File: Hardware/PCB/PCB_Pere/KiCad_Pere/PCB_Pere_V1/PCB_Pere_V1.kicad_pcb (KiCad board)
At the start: 4 copper layers, 52.9 x 80.1 mm, 88 parts, among them CN1 B2B-PH-K-S-GW, CN3 B4B-PH-K-S, CN4 B4B-PH-K-S, U2 TMC2209-LA-T, U3 Buck LMR51625, U4 8132H-10.000NL33DTL, U5 Buck LMR51625, U6 8132H-10.000NL33DTL, U7 TMC2209-LA-T

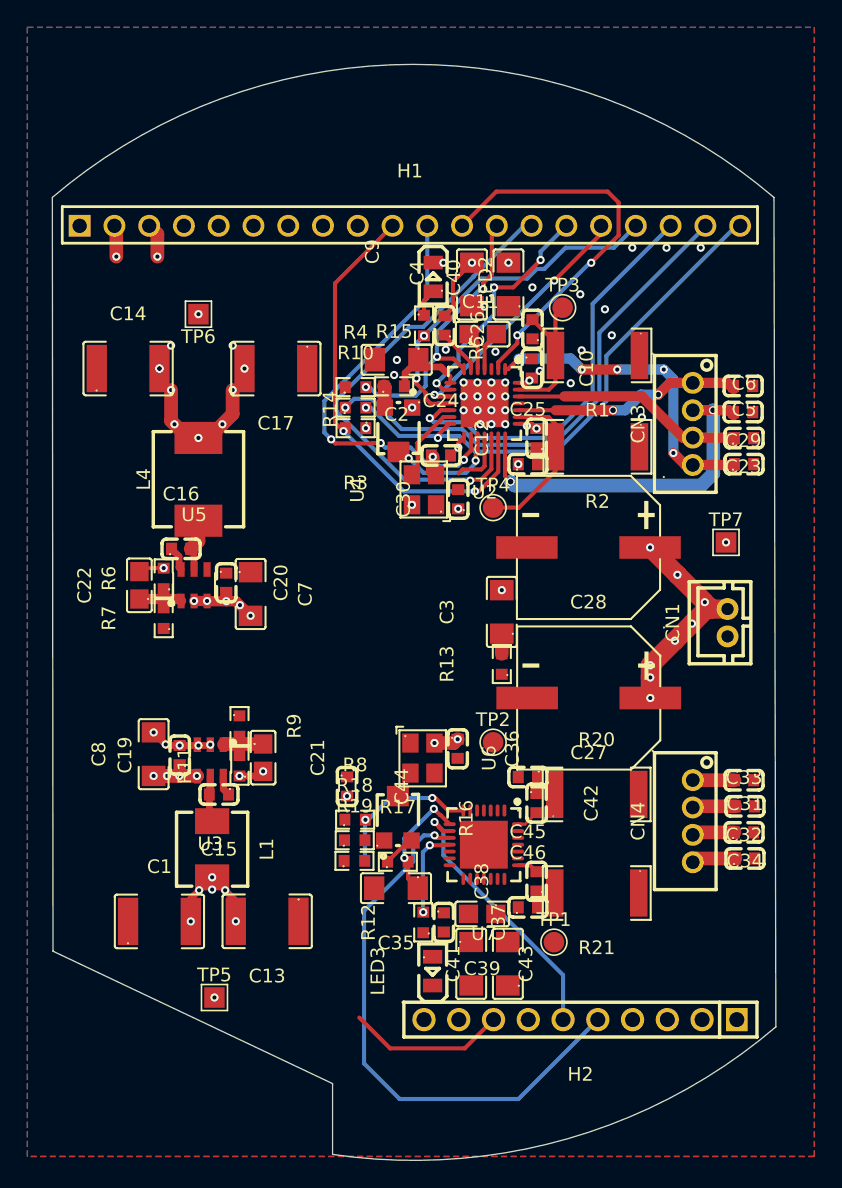
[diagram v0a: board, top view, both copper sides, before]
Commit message: pcb père quasi fini
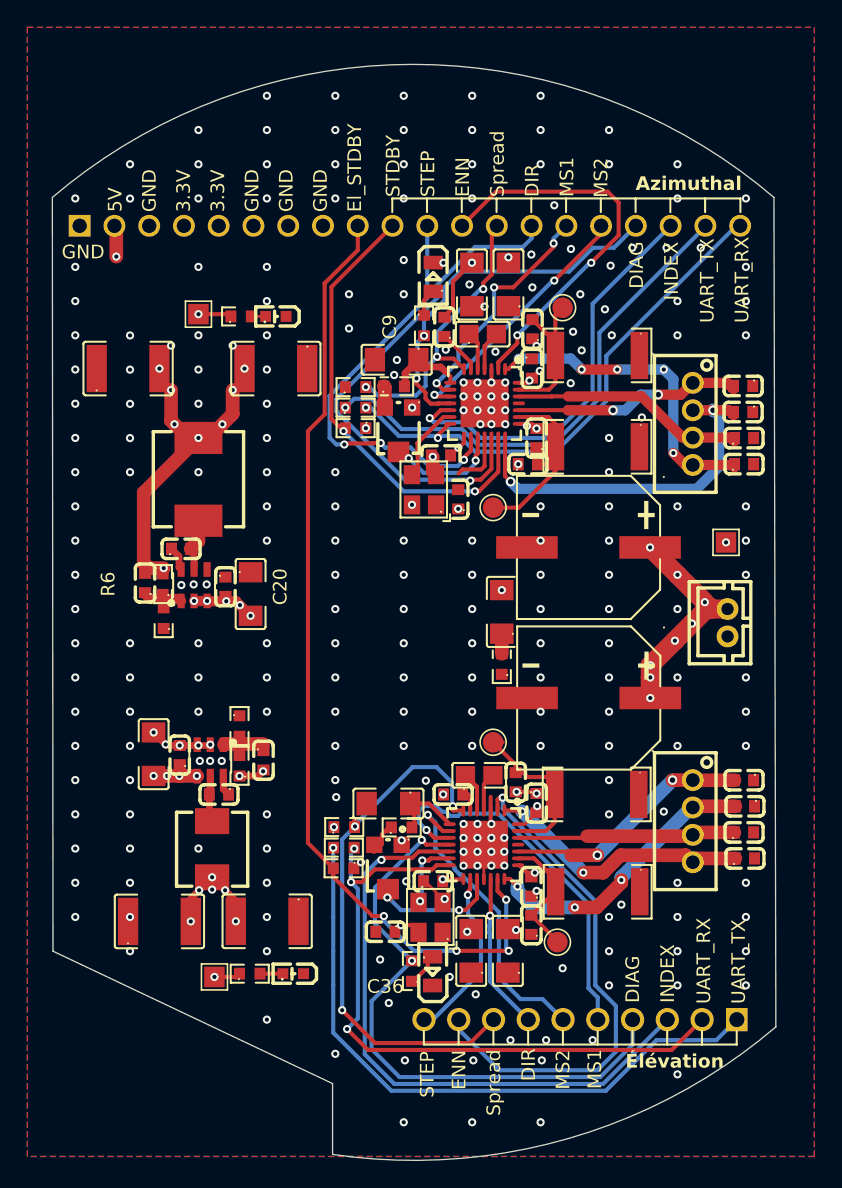
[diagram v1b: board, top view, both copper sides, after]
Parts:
- removed C22: 22nF, EasyEDA:C0805
- added C18: CL10C220JB8NNNC, EasyEDA:C0603, F.Cu at (159.8, 103.5)
- added G***: LOGO, EasyEDA:Logo_astrolab, B.Cu at (182.4, 94.0)
- added LED5: Rouge, EasyEDA:LED-SMD_L1.6-W0.8-R-RD, F.Cu at (160.7, 71.1)
- added LED6: Rouge, EasyEDA:LED-SMD_L1.6-W0.8-R-RD, F.Cu at (161.9, 119.1)
- added R22: 1KΩ, EasyEDA:R0603, F.Cu at (158.1, 71.1)
- added R23: 680, EasyEDA:R0603, F.Cu at (158.8, 119.1)
- C21: value 22nF -> 22pF; footprint EasyEDA:C0805 -> EasyEDA:C0603
- H1, H2: moved to B.Cu
- moved C21 15.4 mm to (151.1, 90.6), turned to 90 degrees
- moved TP2 15.3 mm to (181.2, 116.8)
- moved TP1 15.3 mm to (176.5, 102.2)
- moved C36 14.4 mm to (168.7, 116.1), turned to 180 degrees
- moved U6 11.6 mm to (172.0, 115.0), turned to 90 degrees
- moved C45 10.8 mm to (179.3, 115.6), turned to 90 degrees
- moved C39 10.1 mm to (175.5, 104.6), turned to 0 degrees
- moved C37 9.38 mm to (173.6, 106.0), turned to 180 degrees
- moved C44 9.36 mm to (172.2, 112.4), turned to 0 degrees
- moved C46 9.19 mm to (178.2, 105.2), turned to 90 degrees
- moved R21 7.21 mm to (184.1, 106.0)
- moved R20 7.11 mm to (184.2, 113.2), turned to 180 degrees
- moved C35 6.21 mm to (168.9, 106.7)
- moved R12 3.65 mm to (170.6, 119.0)
- moved R16 3.63 mm to (168.8, 111.3), turned to 90 degrees
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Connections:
- C21 pad 1: /FB_3V3 -> /FB_5V
- C21 pad 2: +3V3 -> +5V
- C23 pad 2: /EL_OA2 -> /AZ_OA2
- C25 pad 2: /Driver Azimutal1/BRB -> /Driver Azimutal1/BRA
- C26 pad 2: /Driver Azimutal1/BRA -> /Driver Azimutal1/BRB
- C29 pad 2: /EL_OA1 -> /AZ_OA1
- C31 pad 1: /AZ_OB2 -> /EL_OB2
- C32 pad 2: /AZ_OA1 -> /EL_OA1
- C33 pad 1: /AZ_OB1 -> /EL_OB1
- C34 pad 2: /AZ_OA2 -> /EL_OA2
- C5 pad 1: /EL_OB2 -> /AZ_OB2
- C6 pad 1: /EL_OB1 -> /AZ_OB1
- CN3 pad 1: /EL_OA1 -> /AZ_OA1
- CN3 pad 2: /EL_OA2 -> /AZ_OA2
- CN3 pad 3: /EL_OB1 -> /AZ_OB1
- CN3 pad 4: /EL_OB2 -> /AZ_OB2
- CN4 pad 1: /AZ_OA1 -> /EL_OA1
- CN4 pad 2: /AZ_OA2 -> /EL_OA2
- CN4 pad 3: /AZ_OB1 -> /EL_OB1
- CN4 pad 4: /AZ_OB2 -> /EL_OB2
- H1 pad 3: +3V3 -> GND
- H1 pad 4: unconnected-(H1-Pad4) -> +3V3
- H1 pad 5: unconnected-(H1-Pad5) -> +3V3
- H1 pad 6: unconnected-(H1-Pad6) -> GND
- H1 pad 7: unconnected-(H1-Pad7) -> GND
- H1 pad 8: unconnected-(H1-Pad8) -> GND
- R1 pad 2: /Driver Azimutal1/BRA -> /Driver Azimutal1/BRB
- R2 pad 2: /Driver Azimutal1/BRB -> /Driver Azimutal1/BRA
- U2 pad 1: /EL_OB2 -> /AZ_OB2
- U2 pad 21: /EL_OA2 -> /AZ_OA2
- U2 pad 23: /Driver Azimutal1/BRB -> /Driver Azimutal1/BRA
- U2 pad 24: /EL_OA1 -> /AZ_OA1
- U2 pad 26: /EL_OB1 -> /AZ_OB1
- U2 pad 27: /Driver Azimutal1/BRA -> /Driver Azimutal1/BRB
- U7 pad 1: /AZ_OB2 -> /EL_OB2
- U7 pad 21: /AZ_OA2 -> /EL_OA2
- U7 pad 24: /AZ_OA1 -> /EL_OA1
- U7 pad 26: /AZ_OB1 -> /EL_OB1
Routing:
- net /STBY_Elevation: track 0.00 -> 70.7 mm, vias 0 -> 4
- net /Driver Elevation/UART_RX: track 0.00 -> 49.0 mm, vias 0 -> 3
- net /Driver Elevation/UART_TX: track 0.00 -> 47.7 mm, vias 0 -> 1
- net /Driver Elevation/Index: track 0.00 -> 45.0 mm, vias 0 -> 1
- net /Driver Elevation/DIAG: track 6.57 -> 43.9 mm
- net /Driver Elevation/ENN: track 0.00 -> 37.2 mm, vias 0 -> 1
- net /AZ_OA2: track 3.15 -> 26.9 mm, vias 0 -> 2
- net /AZ_OB2: track 3.22 -> 23.5 mm, vias 0 -> 5
- net /Driver Elevation/Spread: track 22.7 -> 38.9 mm, vias 2 -> 3
- net /AZ_OB1: track 3.12 -> 17.1 mm
- net /AZ_OA1: track 3.05 -> 16.7 mm, vias 0 -> 2
- net /Driver Elevation/MS2: track 41.0 -> 28.0 mm
- net +5V: track 13.9 -> 26.9 mm, vias 13 -> 12
- net /Driver Elevation/STEP: track 0.00 -> 12.9 mm, vias 0 -> 1
- net /Driver Elevation/BRA: track 0.00 -> 12.5 mm
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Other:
- board text added: "3.3V"
- board text added: "5V"
- board text added: "Azimuthal"
- board text added: "DIAG"
- board text added: "DIR"
- board text added: "ENN"
- board text added: "El_STDBY"
- board text added: "GND"
- board text added: "INDEX"
- board text added: "MS1"
- board text added: "MS2"
- board text added: "STDBY"
- board text added: "STEP"
- board text added: "Spread"
- board text added: "UART_RX"
- board text added: "UART_TX"
- board text added: "Élévation"
